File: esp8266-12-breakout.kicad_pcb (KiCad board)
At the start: 2 copper layers, 32.4 x 39.4 mm, 15 parts, among them P1 ftdi, P2 CONN_01X14, SW1 SW_PUSH, U1 AP1117D33

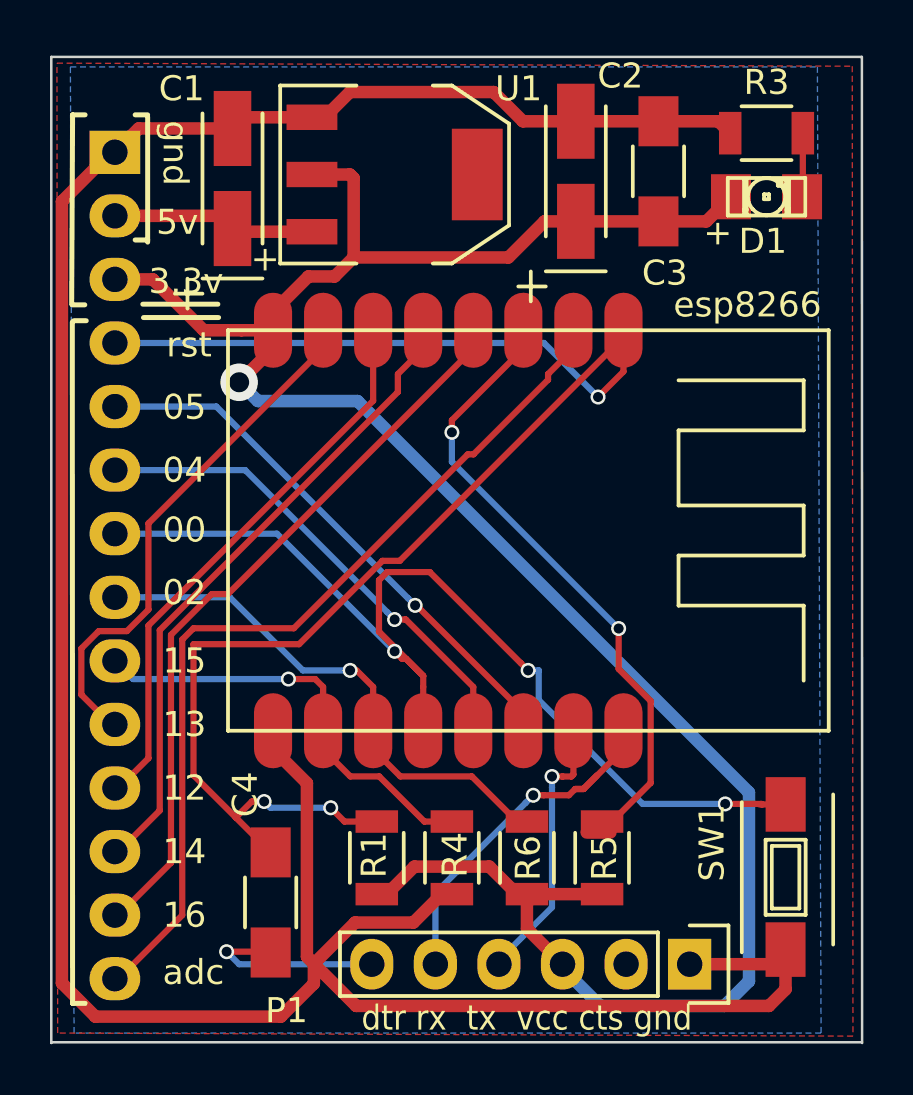
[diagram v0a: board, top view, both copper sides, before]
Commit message: Really strictly align outline
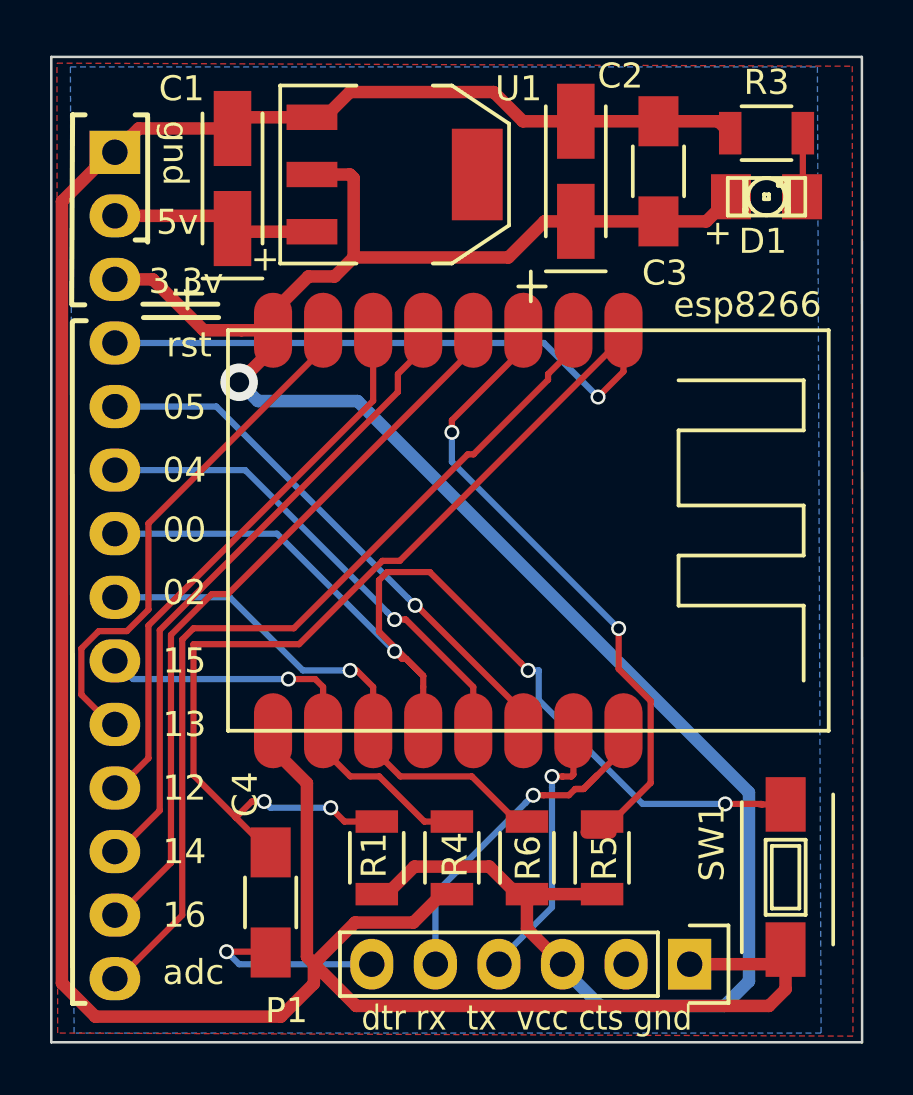
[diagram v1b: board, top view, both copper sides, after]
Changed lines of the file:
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@@
-(kicad_pcb (version 4) (host pcbnew 4.1.0-alpha+201607250104+6992~46~ubuntu14.04.1-product)
+(kicad_pcb (version 4) (host pcbnew 4.0.3+e1-6302~38~ubuntu14.04.1-stable)
   (general
     (links 41)
     (no_connects 0)
-    (area 109.628979 95.9975 142.290001 141.050001)
+    (area 109.628979 95.98 142.290001 141.020001)
     (thickness 1.6)
     (drawings 621)
@@
     (visible_elements FFFEFF7F)
     (pcbplotparams
-      (layerselection 0x010f0_ffffffff)
+      (layerselection 0x010f0_80000001)
       (usegerberextensions false)
       (excludeedgelayer true)
@@
       (hpglpenspeed 20)
       (hpglpendiameter 15)
+      (hpglpenoverlay 2)
       (psnegative false)
       (psa4output false)
@@
     (descr "Through hole pin header")
     (tags "pin header")
-    (fp_text reference P1 (at 1.85 16.106 180) (layer F.SilkS)
+    (fp_text reference P1 (at 1.85 16.106 540) (layer F.SilkS)
       (effects (font (size 1 1) (thickness 0.15)))
     )
@@
     (tags "capacitor 1206")
     (attr smd)
-    (fp_text reference C3 (at -4.064 0.254) (layer F.SilkS)
+    (fp_text reference C3 (at -4.064 0.254 360) (layer F.SilkS)
       (effects (font (size 1 1) (thickness 0.15)))
     )
@@
     (tags "CMS SOT")
     (attr smd)
-    (fp_text reference U1 (at -3.429 -4.953) (layer F.SilkS)
+    (fp_text reference U1 (at -3.429 -4.953 360) (layer F.SilkS)
       (effects (font (size 1 1) (thickness 0.15)))
     )
@@
     (tags "SPST button tactile switch")
     (attr smd)
-    (fp_text reference SW1 (at -1.366 2.942 90) (layer F.SilkS)
+    (fp_text reference SW1 (at -1.366 2.942 450) (layer F.SilkS)
       (effects (font (size 1 1) (thickness 0.15)))
     )
@@
   )
   (gr_line (start 142.24 101.6) (end 109.855 101.6) (layer Edge.Cuts) (width 0.1))
-  (gr_line (start 142.25 141) (end 142.24 101.6) (layer Edge.Cuts) (width 0.1))
+  (gr_line (start 142.25 140.97) (end 142.24 101.6) (layer Edge.Cuts) (width 0.1))
   (gr_line (start 109.855 140.97) (end 142.24 140.97) (layer Edge.Cuts) (width 0.1))
-  (gr_line (start 109.855 101.6) (end 109.855 141) (layer Edge.Cuts) (width 0.1))
+  (gr_line (start 109.855 101.6) (end 109.855 140.97) (layer Edge.Cuts) (width 0.1))
   (segment (start 125.859 135.05) (end 125.459 135.05) (width 0.5) (layer F.Cu) (net 1))
   (segment (start 125.459 135.05) (end 124.32501 136.18399) (width 0.5) (layer F.Cu) (net 1))
